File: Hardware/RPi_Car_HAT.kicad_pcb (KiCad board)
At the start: 2 copper layers, 65 x 56 mm, 44 parts, among them J1 Conn_01x04, J2 Conn_01x02, J3 40HAT, J4 USB_A, Q1 2N3904, Q2 2N3904, Q3 2N3904, Q4 IRF9540N, U1 PC817, U2 PC817, U3 LM10, U4 YAAJ_DCDC_StepDown_LM2596

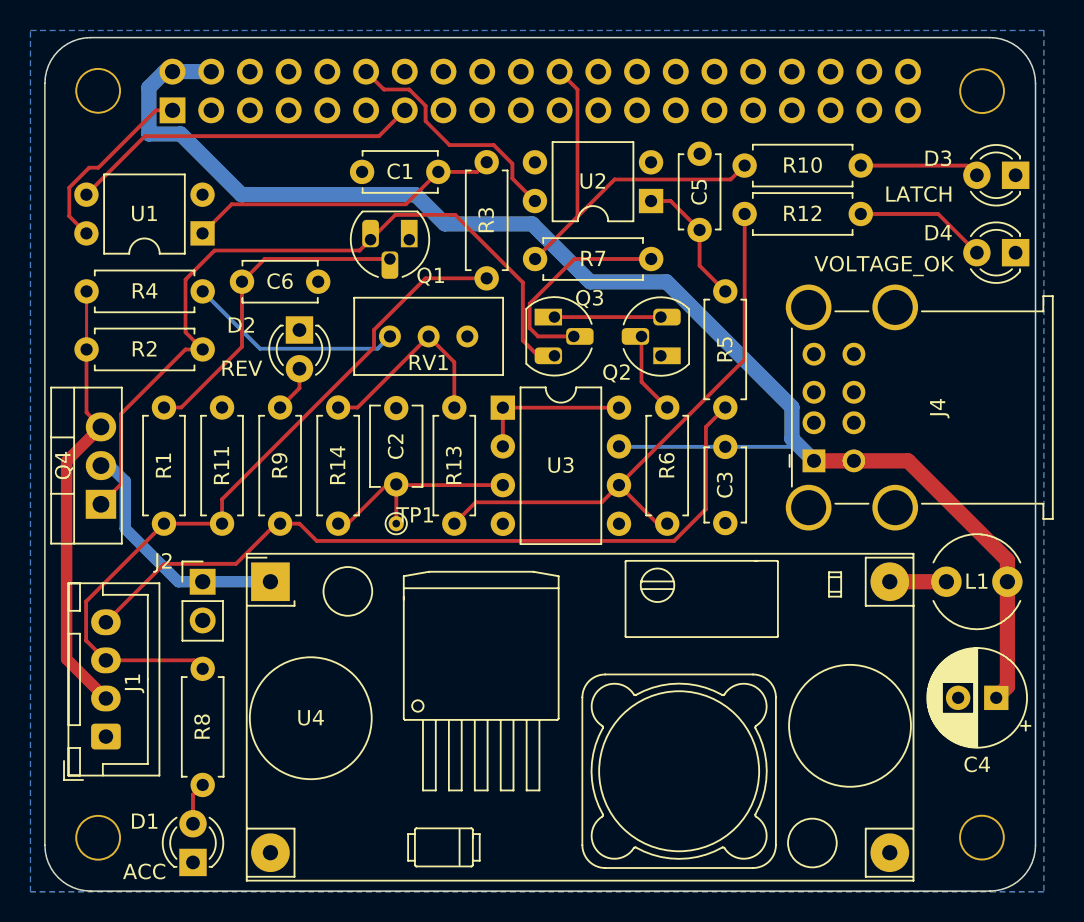
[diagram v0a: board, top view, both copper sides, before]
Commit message: Put ACC trigger behind low voltage cut-off, update to new KiCAD version
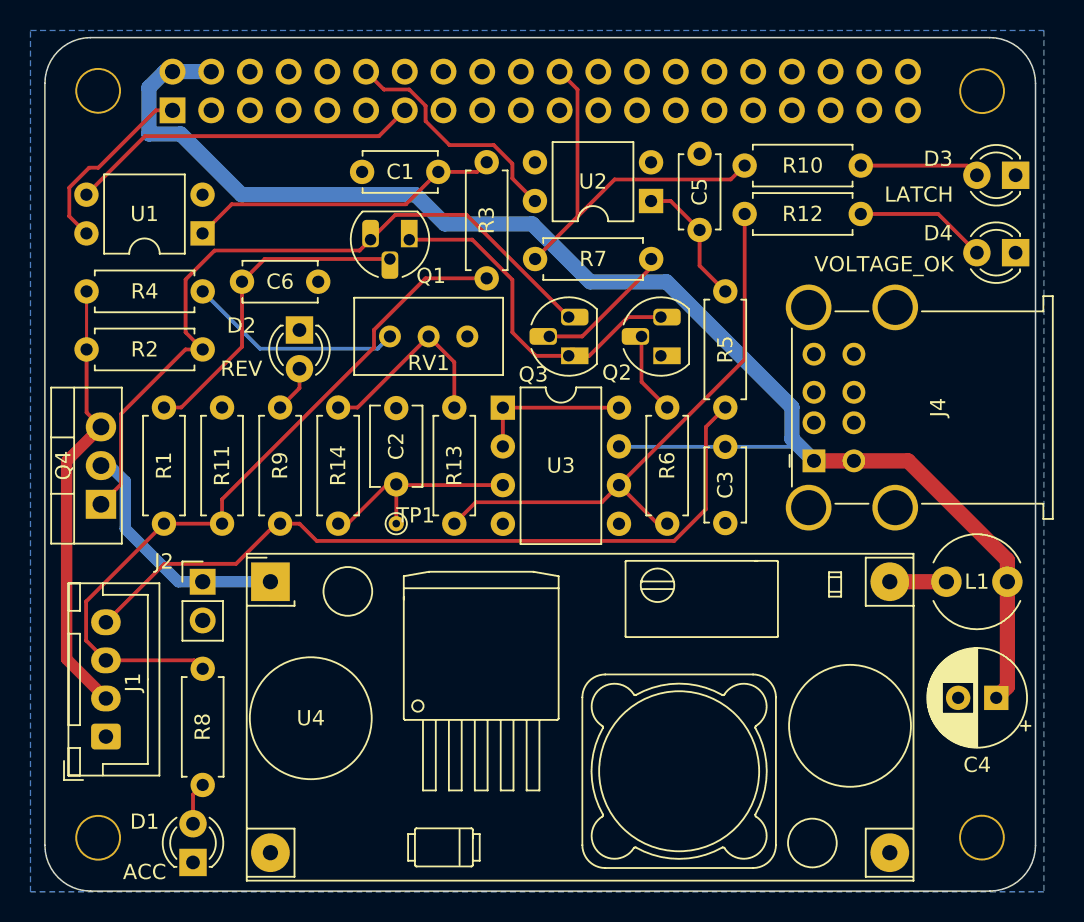
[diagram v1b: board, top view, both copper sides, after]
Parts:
- moved Q3 2.71 mm to (112.9, 81.7), turned to 90 degrees
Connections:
- Q1 pad 1: GND -> Net-(Q1-E)
- Q2 pad 3: Net-(Q2-Pad3) -> Net-(Q1-E)
- Q3 pad 1: Net-(Q2-Pad3) -> Net-(Q1-E)
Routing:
- net Net-(Q1-E): track 0.00 -> 23.0 mm
- net Net-(Q2-Pad3): track 6.98 -> 0.00 mm
- net Net-(Q3-B): track 13.9 -> 9.11 mm
- net Net-(Q1-C): track 50.7 -> 48.3 mm

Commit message: Revert "Put ACC trigger behind low voltage cut-off, update to new KiCAD version"
This reverts commit 32efec27a2ba4a602edbb2af9725aed434bd226d.
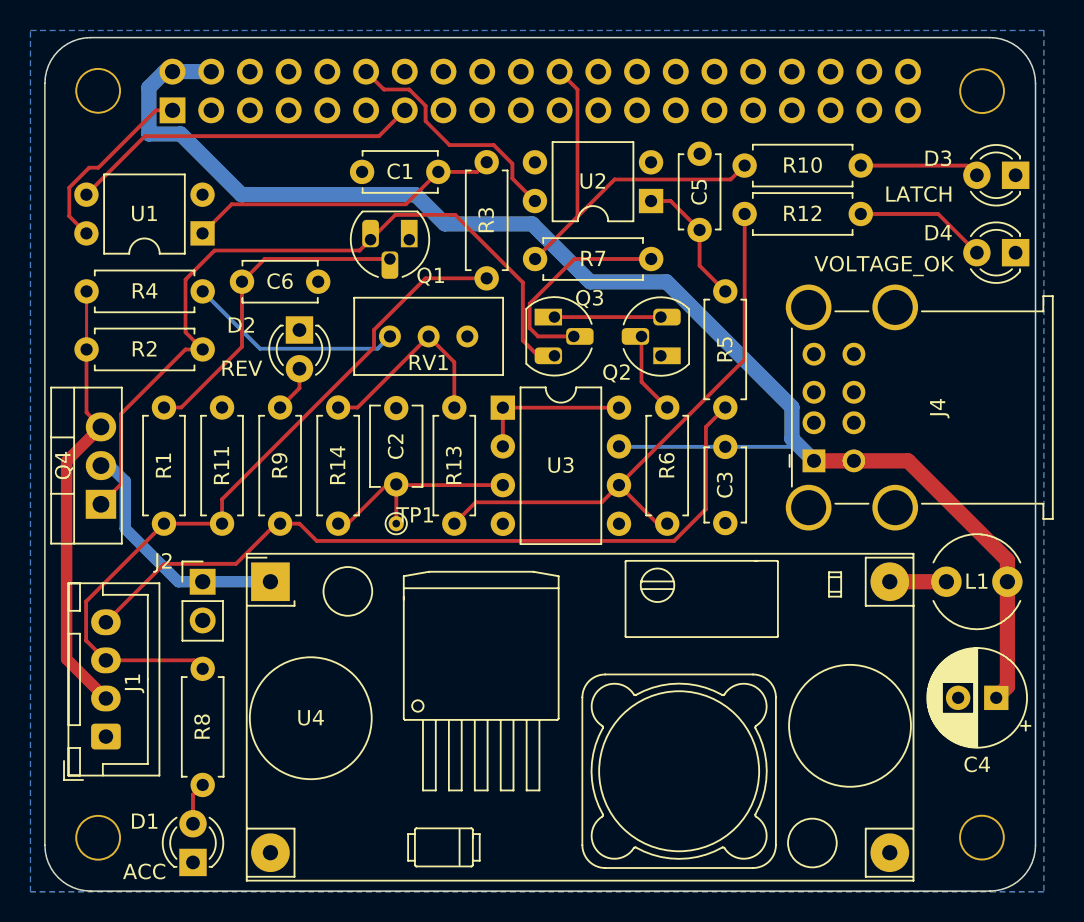
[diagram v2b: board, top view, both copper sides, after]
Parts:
- moved Q3 2.71 mm to (112.0, 79.2), turned to -90 degrees
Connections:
- Q1 pad 1: Net-(Q1-E) -> GND
- Q2 pad 3: Net-(Q1-E) -> Net-(Q2-Pad3)
- Q3 pad 1: Net-(Q1-E) -> Net-(Q2-Pad3)
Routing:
- net Net-(Q1-E): track 23.0 -> 0.00 mm
- net Net-(Q2-Pad3): track 0.00 -> 6.98 mm
- net Net-(Q3-Pad2): track 9.11 -> 13.9 mm
- net Net-(Q1-Pad3): track 48.3 -> 50.7 mm
